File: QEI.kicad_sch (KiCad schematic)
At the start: 21 parts, among them J17 Conn_01x05_Pin, J18 Conn_01x05_Pin, J19 Conn_01x05_Pin

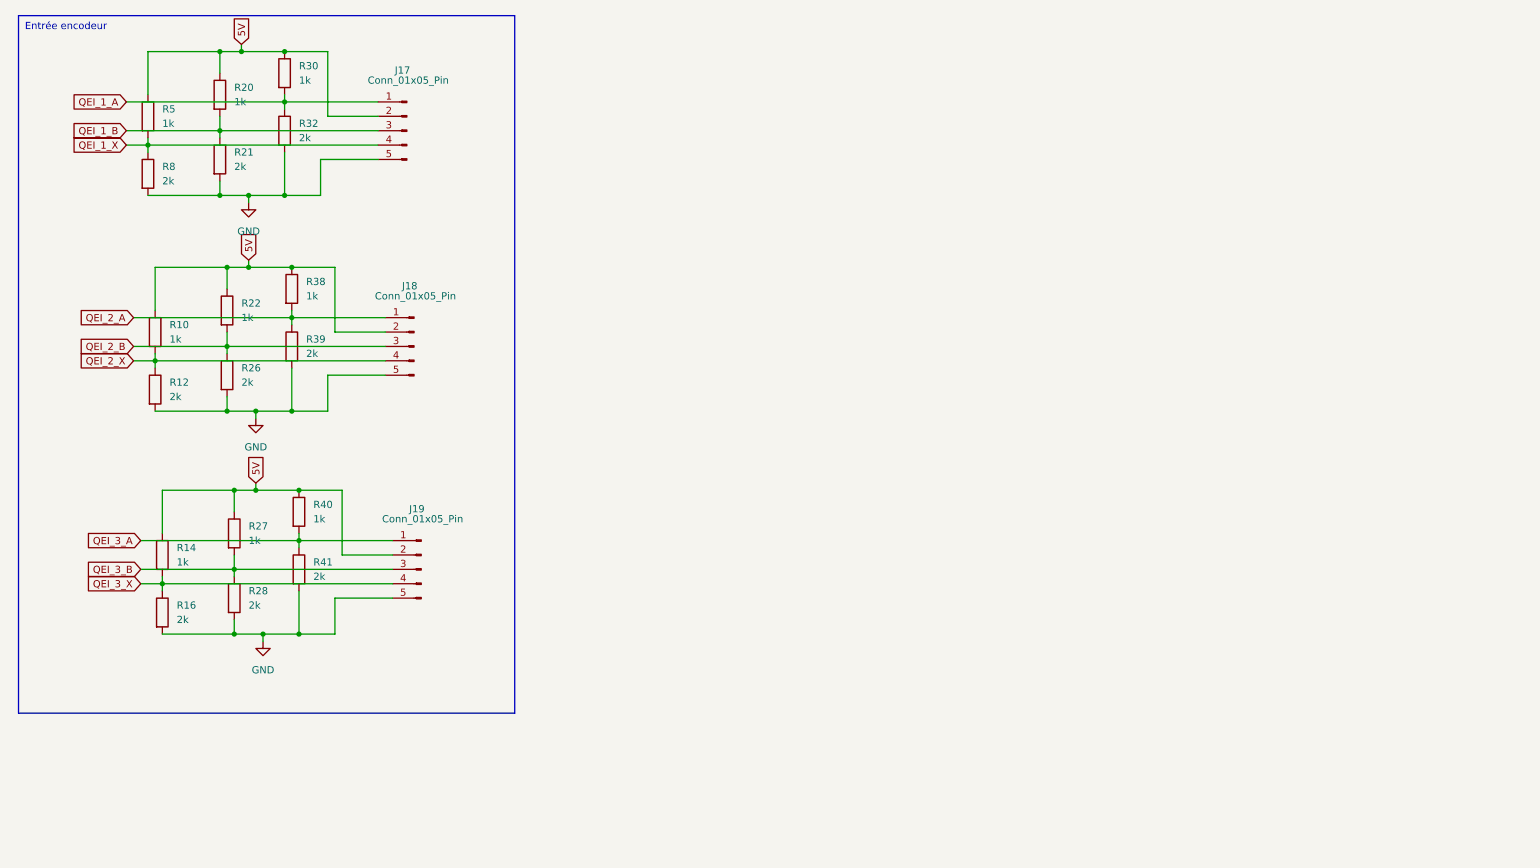
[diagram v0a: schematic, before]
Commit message: fix issues
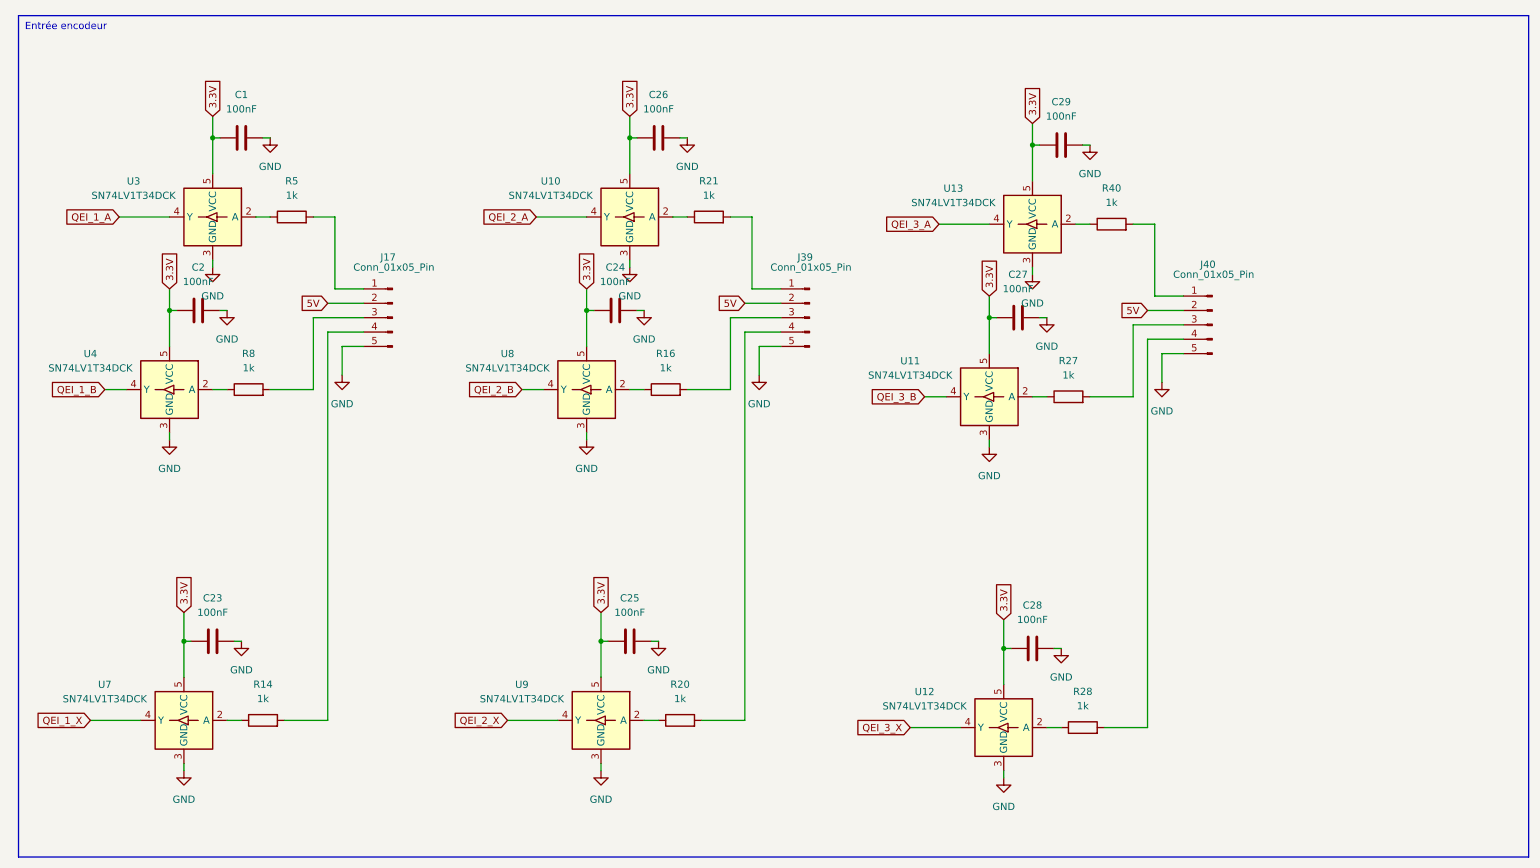
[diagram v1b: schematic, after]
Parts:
- removed J18, J19: Conn_01x05_Pin, Connector_PinHeader_2.54mm:PinHeader_1x05_P2.54mm_Vertical, symbol Connector:Conn_01x05_Pin
- removed R10, R22, R30, R38: 1k, Resistor_SMD:R_0402_1005Metric, symbol Device:R
- removed R12, R26, R32, R39, R41: 2k, Resistor_SMD:R_0402_1005Metric, symbol Device:R
- added C1, C2, C23, C24, C25, C26, C27, C28, C29: 100nF, Capacitor_SMD:C_0402_1005Metric, symbol Device:C
- added J39, J40: Conn_01x05_Pin, Connector_PinHeader_2.54mm:PinHeader_1x05_P2.54mm_Vertical, symbol Connector:Conn_01x05_Pin
- added U10, U11, U12, U13, U3, U4, U7, U8, U9: SN74LV1T34DCK, Package_TO_SOT_SMD:SOT-353_SC-70-5, symbol Logic_LevelTranslator:SN74LV1T34DCK
- R14, R20, R27, R40, R5: footprint Resistor_SMD:R_0402_1005Metric -> Capacitor_SMD:C_0402_1005Metric
- R16, R21, R28, R8: value 2k -> 1k; footprint Resistor_SMD:R_0402_1005Metric -> Capacitor_SMD:C_0402_1005Metric
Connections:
- net 5V: now also J39.2 (Pin_2), J40.2 (Pin_2); no longer R14.1, R20.1, R27.1, R40.1, R5.1
- net GND: now also C1.1, C2.1, C23.1, C24.1, C25.1, C26.1, C27.1, C28.1, C29.1, J39.5 (Pin_5), J40.5 (Pin_5), U10.3 (GND), U11.3 (GND), U12.3 (GND), U13.3 (GND), U3.3 (GND), U4.3 (GND), U7.3 (GND), U8.3 (GND), U9.3 (GND); no longer R16.2, R21.2, R28.2, R8.2
- net QEI_1_A: now also U3.4 (Y); no longer J17.1 (Pin_1)
- net QEI_1_B: now also U4.4 (Y); no longer J17.3 (Pin_3), R20.2, R21.1
- net QEI_1_X: now also U7.4 (Y); no longer J17.4 (Pin_4), R5.2, R8.1
- net QEI_2_A: now also U10.4 (Y)
- net QEI_2_B: now also U8.4 (Y)
- net QEI_2_X: now also U9.4 (Y)
- net QEI_3_A: now also U13.4 (Y); no longer R40.2
- net QEI_3_B: now also U11.4 (Y); no longer R27.2, R28.1
- net QEI_3_X: now also U12.4 (Y); no longer R14.2, R16.1
- new net: R14.1, U7.2 (A)
- new net: R5.1, U3.2 (A)
- new net: J17.1 (Pin_1), R5.2
- new net: R20.1, U9.2 (A)
- new net: J39.4 (Pin_4), R20.2
- new net: R8.1, U4.2 (A)
- new net: R16.1, U8.2 (A)
- new net: R40.1, U13.2 (A)
- new net: R27.1, U11.2 (A)
- new net: J40.3 (Pin_3), R27.2
- new net: J39.3 (Pin_3), R16.2
- new net: R21.1, U10.2 (A)
- new net: J40.1 (Pin_1), R40.2
- new net: J40.4 (Pin_4), R28.2
- new net: J39.1 (Pin_1), R21.2
- new net: J17.3 (Pin_3), R8.2
- new net: J17.4 (Pin_4), R14.2
- new net: R28.1, U12.2 (A)
- new net 3.3V: C1.2, C2.2, C23.2, C24.2, C25.2, C26.2, C27.2, C28.2, C29.2, U10.5 (VCC), U11.5 (VCC), U12.5 (VCC), U13.5 (VCC), U3.5 (VCC), U4.5 (VCC), U7.5 (VCC), U8.5 (VCC), U9.5 (VCC)
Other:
- moved on the sheet: J17

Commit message: update
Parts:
- J17, J39, J40: now left out of the parts list
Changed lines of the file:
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@@
 		(unit 1)
 		(exclude_from_sim no)
-		(in_bom yes)
+		(in_bom no)
 		(on_board yes)
 		(dnp no)
@@
 		(unit 1)
 		(exclude_from_sim no)
-		(in_bom yes)
+		(in_bom no)
 		(on_board yes)
 		(dnp no)
@@
 		(unit 1)
 		(exclude_from_sim no)
-		(in_bom yes)
-		(on_board yes)
-		(dnp no)
+		(in_bom no)
+		(on_board yes)
+		(dnp no)
